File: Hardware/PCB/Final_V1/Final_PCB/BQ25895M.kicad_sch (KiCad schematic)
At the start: 40 parts, among them IC1 BQ25895MRTWT

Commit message: #4: Layout-Session-17-11-25
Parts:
- BT1: footprint (none) -> Connector_PinHeader_2.54mm:PinHeader_1x02_P2.54mm_Vertical
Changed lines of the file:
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@@
 			)
 		)
-		(property "Footprint" ""
+		(property "Footprint" "Connector_PinHeader_2.54mm:PinHeader_1x02_P2.54mm_Vertical"
 			(at 184.15 101.346 90)
 			(effects

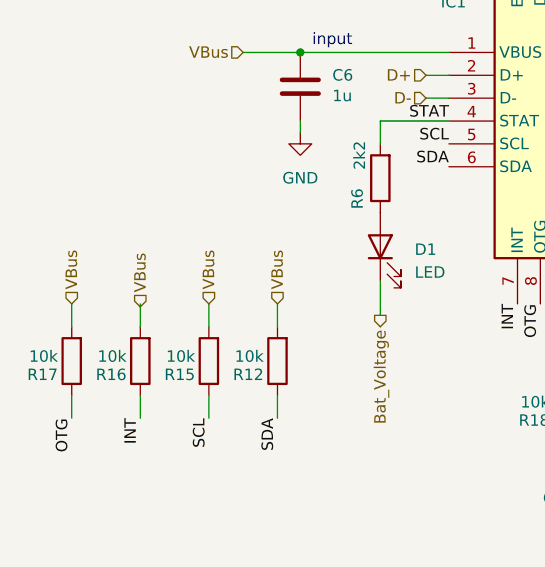
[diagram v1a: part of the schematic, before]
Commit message: a few pcb edits
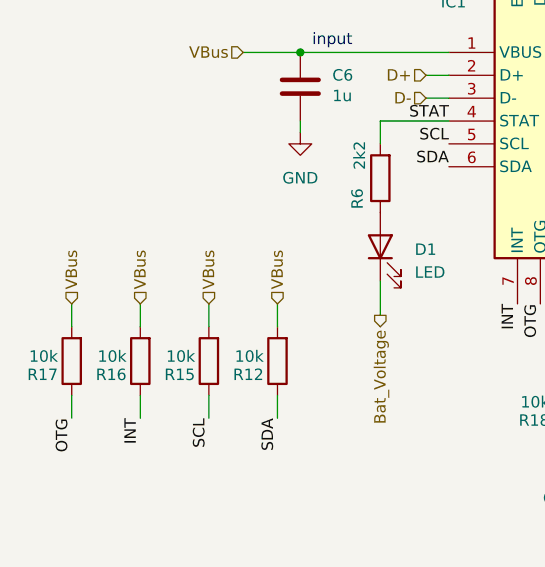
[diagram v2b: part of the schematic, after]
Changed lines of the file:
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@@
-	(wire
-		(pts
-			(xy 81.28 115.57) (xy 81.28 113.03)
-		)
-		(stroke
-			(width 0)
-			(type default)
-		)
-	)
 	(wire
 		(pts
@@
 		(pts
 			(xy 124.46 34.29) (xy 124.46 29.21)
+		)
+		(stroke
+			(width 0)
+			(type default)
+		)
+	)
+	(wire
+		(pts
+			(xy 81.28 113.03) (xy 81.28 115.57)
 		)
 		(stroke
@@
 	(hierarchical_label "VBus"
 		(shape input)
-		(at 81.28 113.3627 90)
-		(effects
-			(font
+		(at 81.28 113.03 90)
+		(effects
+			(font
